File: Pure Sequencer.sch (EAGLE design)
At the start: 133 parts, among them IC2 TL074, IC3 TL074, IC4 TL074, IC5 ATMEGA328P, IC6 CD4051, Q1 20MHz, T1 MMBT3904, T2 MMBT3904

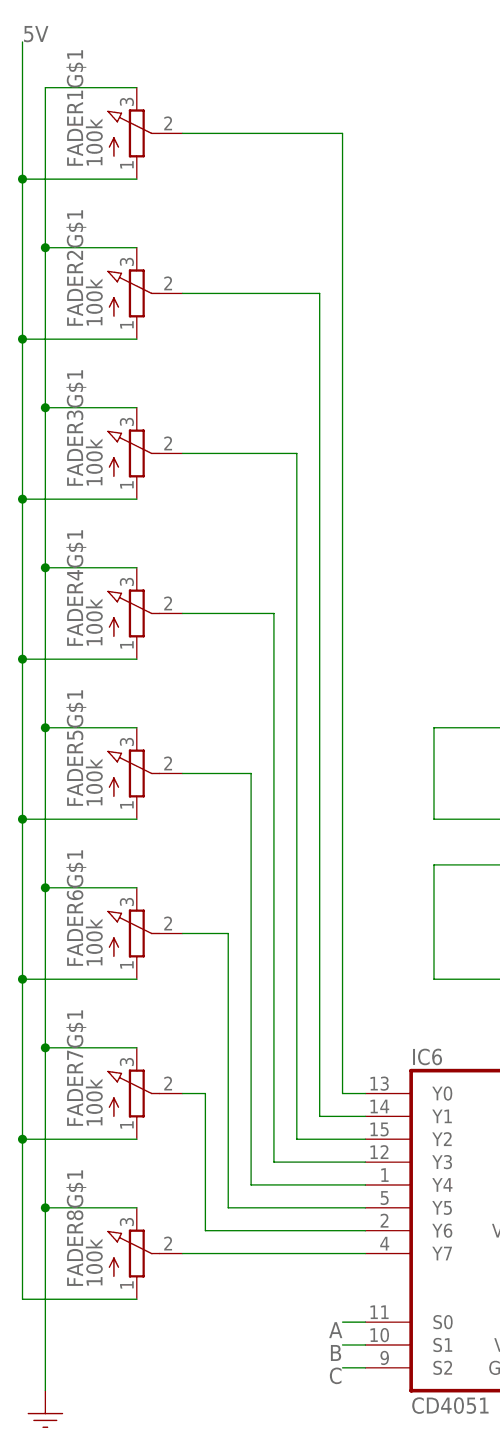
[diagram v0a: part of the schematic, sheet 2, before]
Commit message: Reinstall
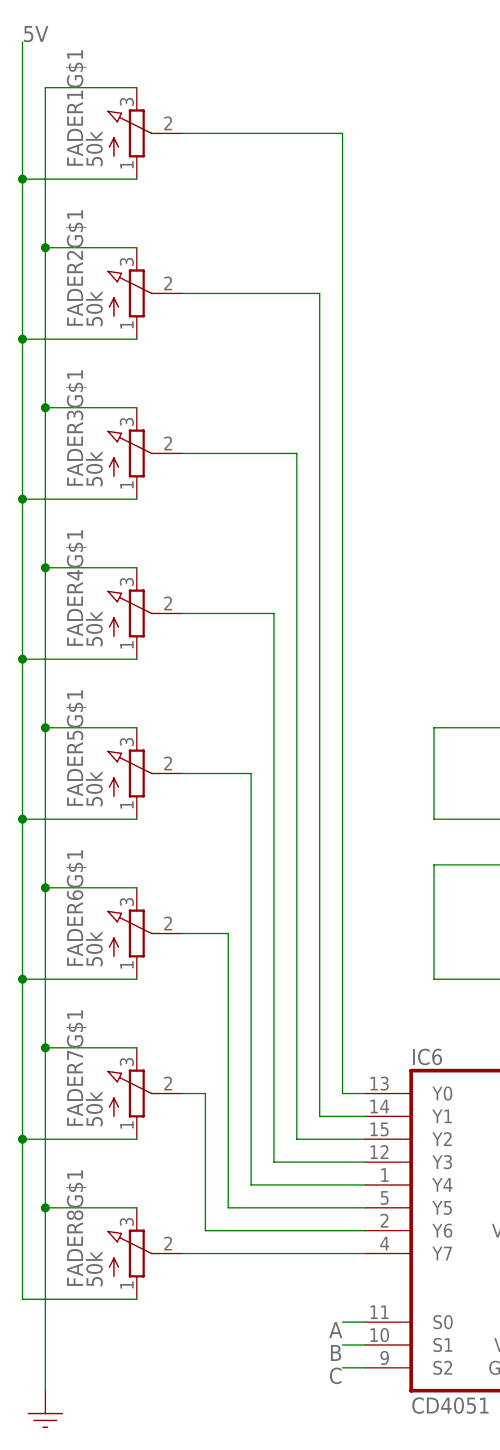
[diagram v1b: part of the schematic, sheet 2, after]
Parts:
- FADER1, FADER2, FADER3, FADER4, FADER5, FADER6, FADER7, FADER8: value 100k -> 50k
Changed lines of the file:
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@@
 <part name="C5" library="GMSN" deviceset="CAPACITOR_POL-US" device="153CLV-0505" value="10uF"/>
 <part name="GND8" library="GMSN" deviceset="GND" device=""/>
-<part name="FADER1" library="GMSN" deviceset="RESISTOR_VARIABLE_LED" device="" value="100k"/>
-<part name="FADER2" library="GMSN" deviceset="RESISTOR_VARIABLE_LED" device="" value="100k"/>
-<part name="FADER3" library="GMSN" deviceset="RESISTOR_VARIABLE_LED" device="" value="100k"/>
-<part name="FADER4" library="GMSN" deviceset="RESISTOR_VARIABLE_LED" device="" value="100k"/>
-<part name="FADER5" library="GMSN" deviceset="RESISTOR_VARIABLE_LED" device="" value="100k"/>
-<part name="FADER6" library="GMSN" deviceset="RESISTOR_VARIABLE_LED" device="" value="100k"/>
-<part name="FADER7" library="GMSN" deviceset="RESISTOR_VARIABLE_LED" device="" value="100k"/>
-<part name="FADER8" library="GMSN" deviceset="RESISTOR_VARIABLE_LED" device="" value="100k"/>
+<part name="FADER1" library="GMSN" deviceset="RESISTOR_VARIABLE_LED" device="" value="50k"/>
+<part name="FADER2" library="GMSN" deviceset="RESISTOR_VARIABLE_LED" device="" value="50k"/>
+<part name="FADER3" library="GMSN" deviceset="RESISTOR_VARIABLE_LED" device="" value="50k"/>
+<part name="FADER4" library="GMSN" deviceset="RESISTOR_VARIABLE_LED" device="" value="50k"/>
+<part name="FADER5" library="GMSN" deviceset="RESISTOR_VARIABLE_LED" device="" value="50k"/>
+<part name="FADER6" library="GMSN" deviceset="RESISTOR_VARIABLE_LED" device="" value="50k"/>
+<part name="FADER7" library="GMSN" deviceset="RESISTOR_VARIABLE_LED" device="" value="50k"/>
+<part name="FADER8" library="GMSN" deviceset="RESISTOR_VARIABLE_LED" device="" value="50k"/>
 <part name="GND4" library="GMSN" deviceset="GND" device=""/>
 <part name="IC6" library="GMSN" deviceset="MUX_1X8_CD4051" device="" value="CD4051"/>
